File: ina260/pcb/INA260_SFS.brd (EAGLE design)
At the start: 85 x 56 mm, 52 parts

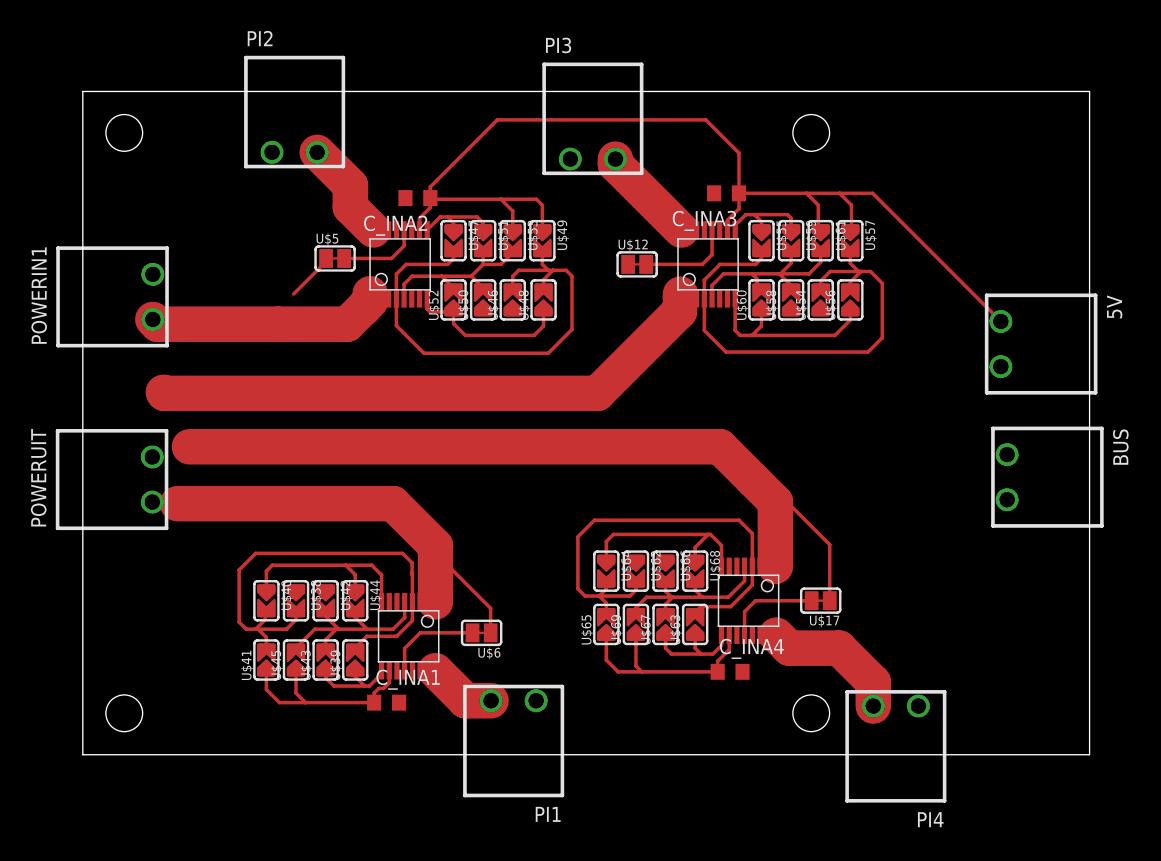
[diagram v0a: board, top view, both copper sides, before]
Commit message: finshed first design. after review ready for order
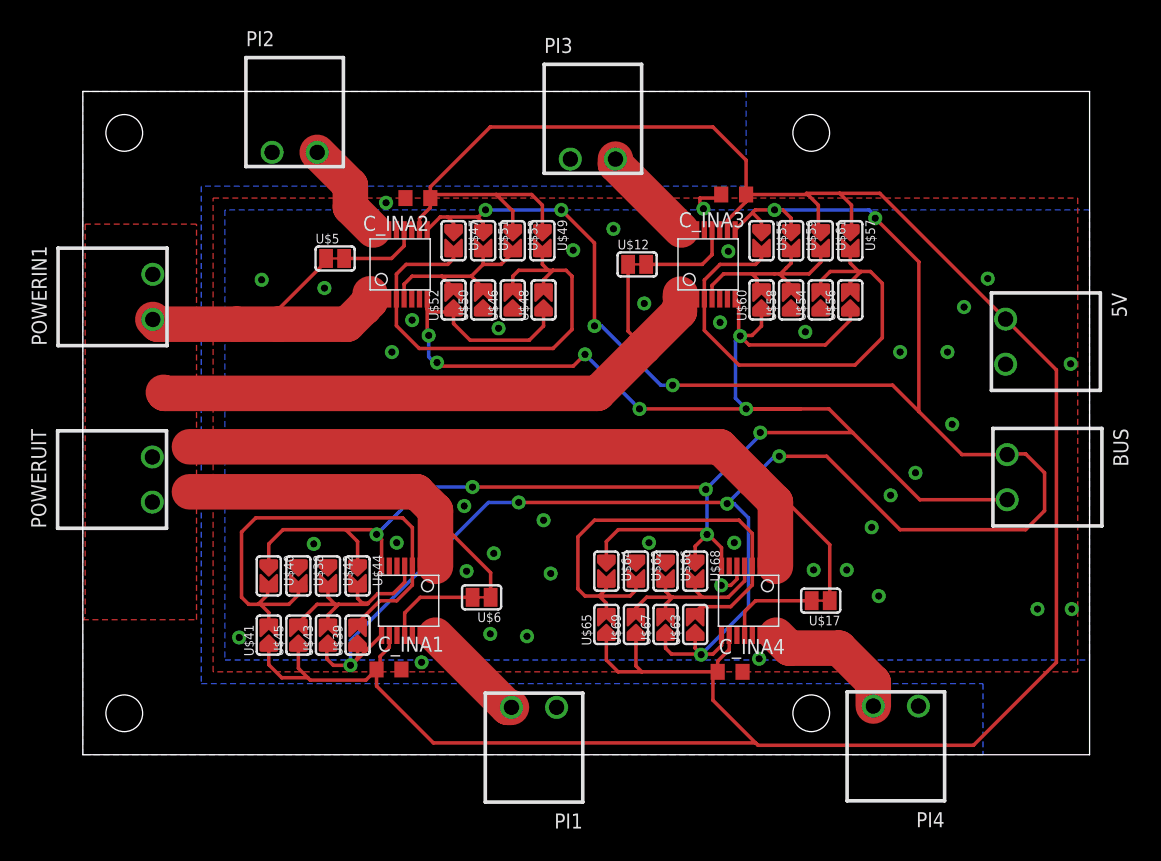
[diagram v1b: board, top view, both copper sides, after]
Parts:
- moved U$1 3.00 mm to (27.5, 13.0)
- moved U$6 3.00 mm to (33.7, 13.3)
- moved C_INA1 2.81 mm to (25.9, 7.20)
- moved U$38 2.11 mm to (18.2, 15.1)
- moved U$39 2.11 mm to (23.2, 10.1)
- moved U$40 2.11 mm to (15.7, 15.1)
- moved U$41 2.11 mm to (15.7, 10.1)
- moved U$42 2.11 mm to (20.7, 15.1)
- moved U$43 2.11 mm to (20.7, 10.1)
- moved U$44 2.11 mm to (23.2, 15.1)
- moved U$45 2.11 mm to (18.2, 10.1)
- moved PI1 1.81 mm to (40.0, 4.00)
- moved C_INA3 0.61 mm to (54.9, 47.3)
- moved 5V 0.45 mm to (77.9, 36.8)
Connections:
- net SCL: now also BUS.P$1; no longer BUS.P$2
- net SDA: now also BUS.P$2; no longer BUS.P$1
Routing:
- net SCL: track 31.5 -> 211.1 mm, vias 0 -> 11
- net SDA: track 62.3 -> 185.0 mm, vias 0 -> 11
- net +5V: track 125.7 -> 229.3 mm
- net IN+: track 179.9 -> 199.9 mm
- net GND: track 0.00 -> 5.57 mm, vias 0 -> 42
- net IN-_1: track 5.75 -> 10.2 mm
- net IN-_4: track 11.8 -> 13.2 mm
- net IN-_3: track 8.29 -> 9.59 mm
- net A1_INA3: track 41.4 -> 42.3 mm
- net A1_INA1: track 40.4 -> 41.2 mm
- added copper zone on layer 1, net GND
- added copper zone on layer 16, net GND
- added copper zone on layer 1, net IN+
